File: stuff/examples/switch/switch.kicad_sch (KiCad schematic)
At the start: 3 parts

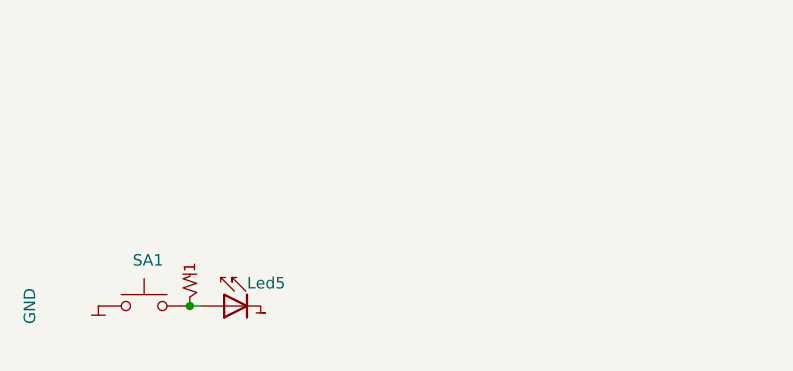
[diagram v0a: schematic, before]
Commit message: - some fixme
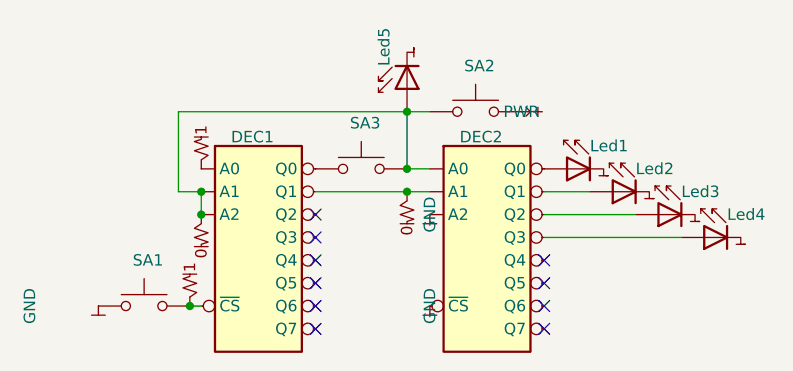
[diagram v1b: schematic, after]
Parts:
- added DEC1, DEC2: decode_3_bit, symbol chip:DECODE_3BIT
- added Led1, Led2, Led3, Led4: ~, symbol chip:LED
- added SA2, SA3: SW_Push, symbol Switch:SW_Push
- added pulldown1, pulldown2: pull_down, symbol chip:PULLDOWN
- added pullup1: pull_up, symbol chip:PULLUP
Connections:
- net gnd: now also DEC2.12 (~{CS}), DEC2.3 (A2)
- net at SA1.2, pullup2.1 (OUT): now also DEC1.12 (~{CS}); no longer Led5.1 (IN)
- new net: DEC2.5 (Q1), Led2.1 (IN)
- new net: DEC1.2 (A1), DEC1.3 (A2), DEC2.1 (A0), Led5.1 (IN), SA2.1, SA3.2, pulldown1.1 (OUT)
- new net: DEC1.1 (A0), pullup1.1 (OUT)
- new net: DEC1.5 (Q1), DEC2.2 (A1), pulldown2.1 (OUT)
- new net: DEC2.4 (Q0), Led1.1 (IN)
- new net: DEC2.6 (Q2), Led3.1 (IN)
- new net: DEC2.7 (Q3), Led4.1 (IN)
- new net: DEC1.4 (Q0), SA3.1
- new net pwr: SA2.2
- no-connect marks 0 -> 10
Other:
- moved on the sheet: Led5
